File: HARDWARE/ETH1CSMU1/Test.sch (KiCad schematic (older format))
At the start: 27 parts, among them U1601 OPA2344, U1602 OPA2344, U1603 PCA9536D, U1604 DG408DY, U1605 OPA344, U1606 ADS1110, U1607 AD8628

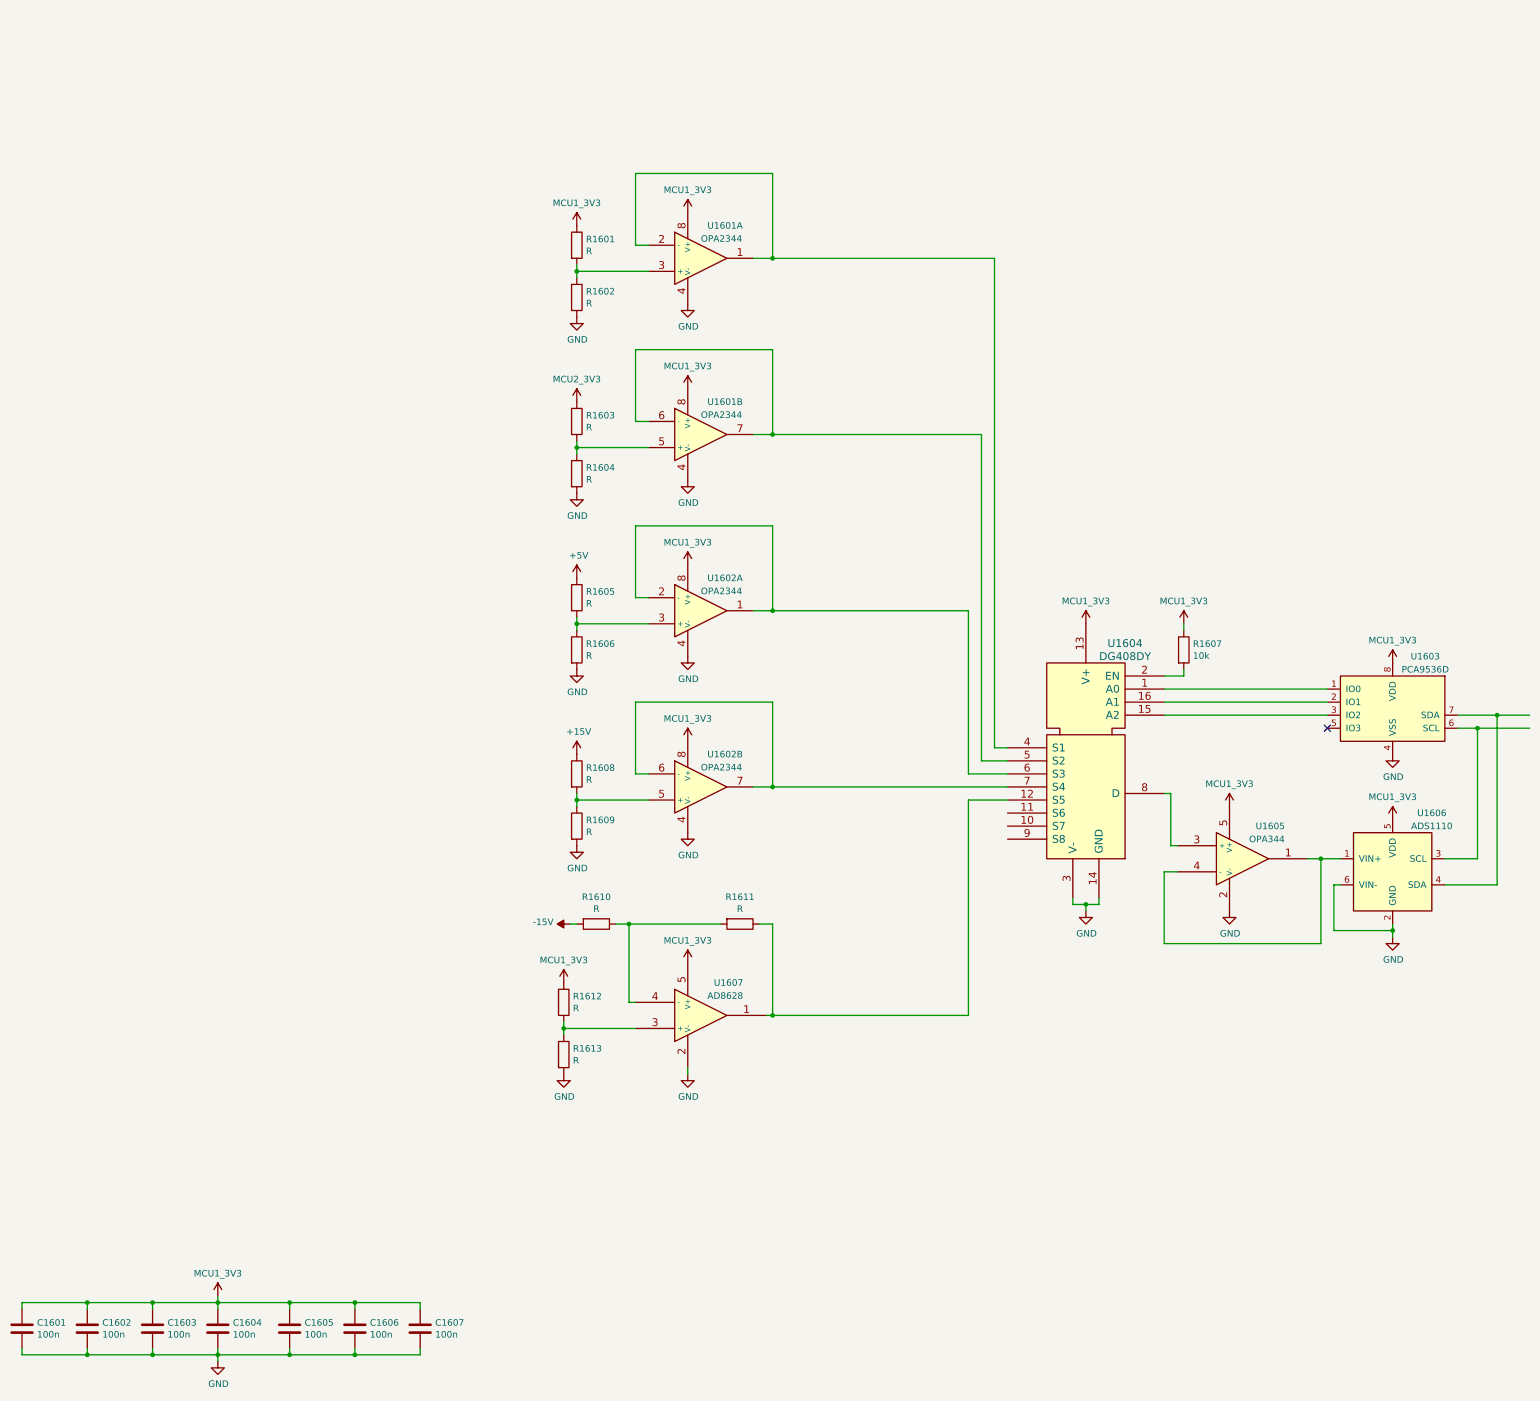
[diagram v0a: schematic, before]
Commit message: Bug fix
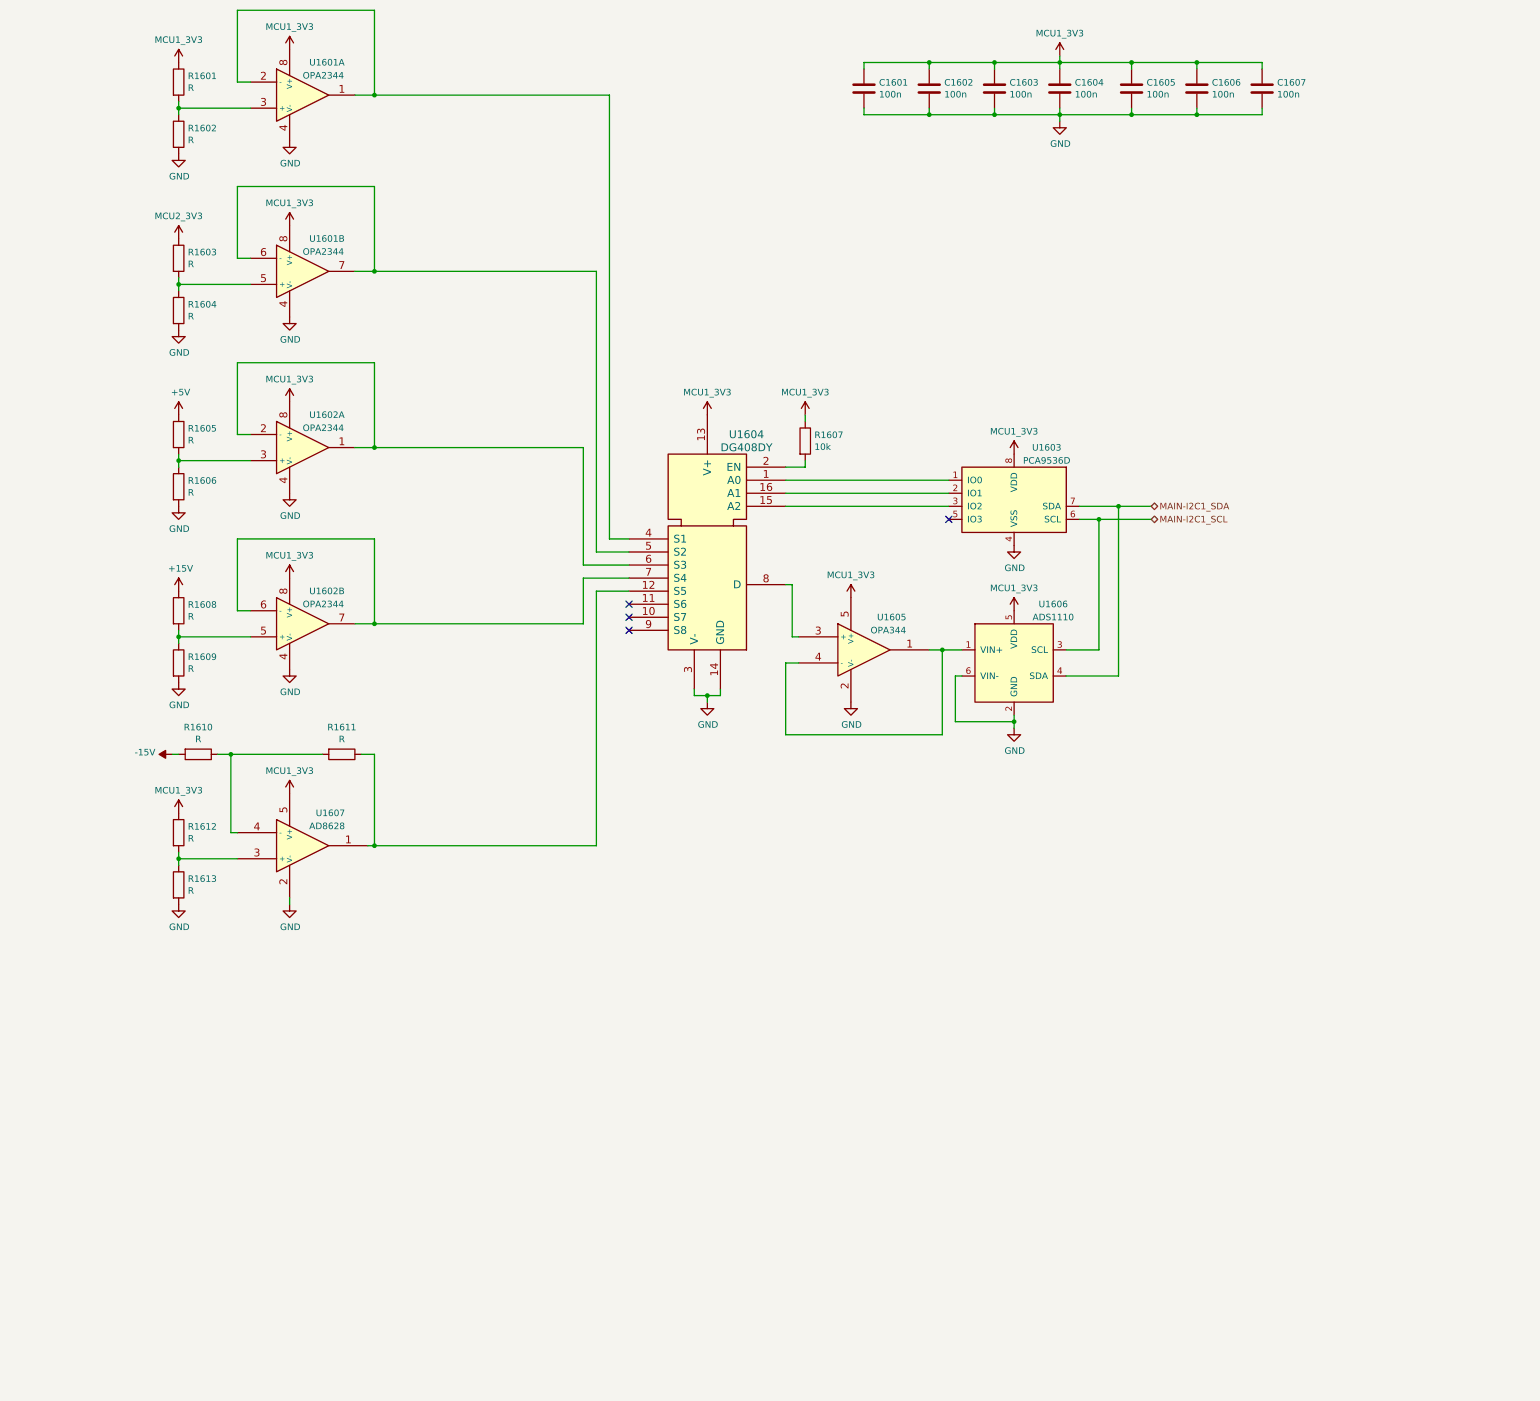
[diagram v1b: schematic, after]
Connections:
- net MAIN-I2C1_SCL: now reaches U1603.6 (SCL), U1606.3 (SCL)
- net MAIN-I2C1_SDA: now reaches U1603.7 (SDA), U1606.4 (SDA)
- no-connect marks 1 -> 4
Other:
- moved on the sheet: C1601, C1602, C1603, C1604, C1605, C1606, C1607, R1601, R1602, R1603, R1604, R1605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
